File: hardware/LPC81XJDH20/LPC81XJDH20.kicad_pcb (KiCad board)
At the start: 2 copper layers, 18.7 x 23.8 mm, 24 parts, among them J1 Conn_01x09, J2 JTAG_2X05, J3 Conn_01x09, U1 LPC824M201JDH20, Y1 12MHz

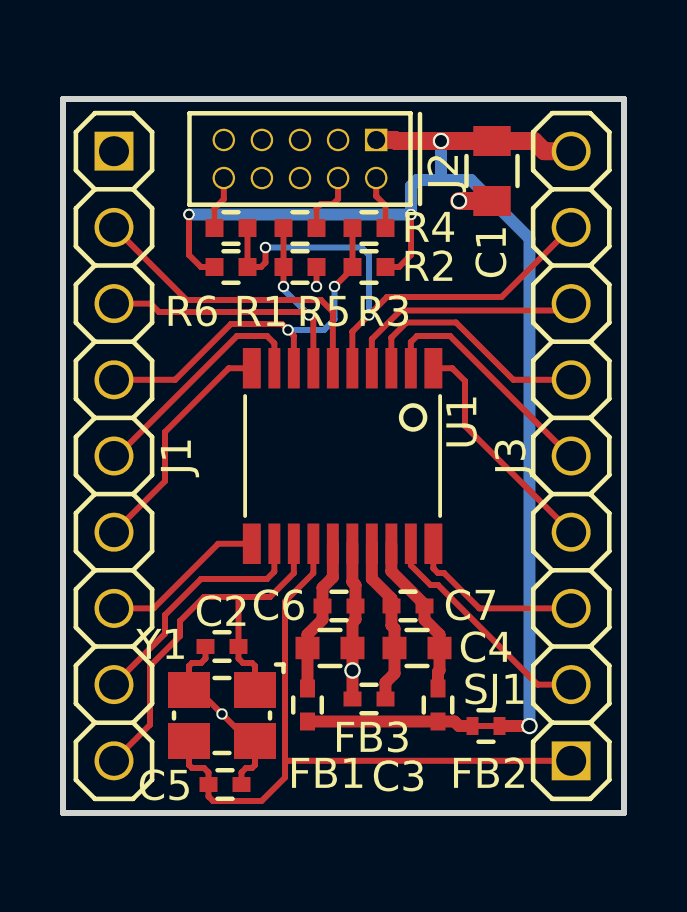
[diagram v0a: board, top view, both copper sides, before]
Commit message: WIP PCB layout
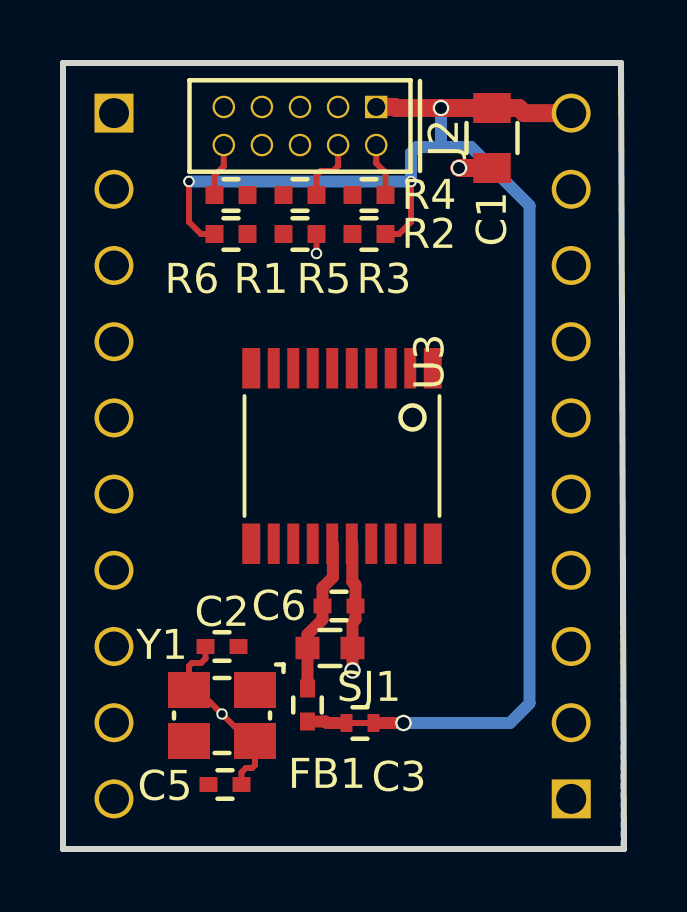
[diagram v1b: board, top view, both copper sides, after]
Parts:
- removed C4: 1u, SquantorRcl:C_0603
- removed C7: 100n, SquantorRcl:C_0402
- removed FB2, FB3: FB, SquantorRcl:C_0402
- removed U1: LPC824M201JDH20, SquantorIC:SOT360
- added U3: LPC812M101JDH20, SquantorIC:SOT360, F.Cu at (134.6, 101.6)
- J1: value Conn_01x09 -> LPC81XJDH20_breakout_left; footprint SquantorConnectors:Header-0254-1X09-H010 -> SquantorConnectorsNamed:LPC81XJDH20_breakout_left; moved to B.Cu
- J3: value Conn_01x09 -> LPC81XJDH20_breakout_right; footprint SquantorConnectors:Header-0254-1X09-H010 -> SquantorConnectorsNamed:LPC81XJDH20_breakout_right; moved to B.Cu
- N2: value 20190121 -> 20190310
- moved SJ1 4.20 mm to (135.2, 110.5)
- moved J2 1.10 mm to (133.2, 90.6)
- moved C1 1.10 mm to (139.6, 91.0)
- moved R1 1.10 mm to (130.9, 94.2)
- moved R2 1.10 mm to (135.5, 94.2)
- moved R3 1.10 mm to (133.2, 94.2)
- moved R4 1.10 mm to (135.5, 92.9)
- moved R5 1.10 mm to (133.2, 92.9)
- moved R6 1.10 mm to (130.9, 92.9)
- turned J3 to 270 degrees
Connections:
- J1 pad 2: /PIO0_4 -> /PIO0_3
- J1 pad 3: /PIO0_3 -> /PIO0_2
- J1 pad 4: /PIO0_2 -> /PIO0_11
- J1 pad 5: /PIO0_11 -> /PIO0_10
- J1 pad 6: /PIO0_10 -> /PIO0_16
- J3 pad 1: /PIO0_8 -> /PIO0_7
- J3 pad 2: /PIO0_0 -> /PIO0_6
- J3 pad 3: /PIO0_14 -> /PIO0_0
- J3 pad 4: /PIO0_23 -> /PIO0_14
- J3 pad 9: VDD -> /PIO0_4
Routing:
- net /PIO0_8: track 23.0 -> 0.00 mm
- net /RESET: track 18.0 -> 0.00 mm, vias 2 -> 0
- net /PIO0_9: track 14.5 -> 0.00 mm
- net /PIO0_2: track 13.0 -> 0.00 mm, vias 2 -> 0
- net /PIO0_3: track 11.7 -> 0.00 mm, vias 2 -> 0
- net /PIO0_4: track 10.3 -> 0.00 mm
- net /PIO0_1: track 8.20 -> 0.00 mm
- net /PIO0_12: track 8.11 -> 0.00 mm
- net /PIO0_13: track 8.02 -> 0.00 mm
- net /PIO0_17: track 7.96 -> 0.00 mm
- net /PIO0_11: track 7.93 -> 0.00 mm
- net /PIO0_10: track 7.82 -> 0.00 mm
- net /PIO0_23: track 7.74 -> 0.00 mm
- net /PIO0_0: track 7.71 -> 0.00 mm
- net /PIO0_14: track 5.97 -> 0.00 mm
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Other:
- board size 18.7 x 23.8 mm -> 18.7 x 26.2 mm
